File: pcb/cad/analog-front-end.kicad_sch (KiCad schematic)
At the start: 30 parts

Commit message: specify components used in front-end, validation and power circuits, except resistors
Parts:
- C?: footprint (none) -> Capacitor_SMD:C_0805_2012Metric_Pad1.18x1.45mm_HandSolder; Manufacturer (none) -> Prosperity Dielectrics Co; Part Number (none) -> MA0805CG-331J-500PR
- R?: footprint Resistor_SMD:R_0603_1608Metric -> Resistor_SMD:R_0603_1608Metric_Pad0.98x0.95mm_HandSolder; Vendor Link (none) -> https://www.digikey.com/en/products/detail/ERA-3AEB473V/P47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
- RV?: footprint (none) -> Potentiometer_SMD:Potentiometer_Bourns_3224X_Vertical; Manufacturer (none) -> Bourns; Part Number (none) -> 3224X-1-502E
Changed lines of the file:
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@@
       (effects (font (size 1.27 1.27)) (justify left))
     )
-    (property "Footprint" "" (id 2) (at 100.0252 67.31 0)
-      (effects (font (size 1.27 1.27)) hide)
-    )
-    (property "Datasheet" "~" (id 3) (at 99.06 63.5 0)
+    (property "Footprint" "Capacitor_SMD:C_0805_2012Metric_Pad1.18x1.45mm_HandSolder" (id 2) (at 100.0252 67.31 0)
+      (effects (font (size 1.27 1.27)) hide)
+    )
+    (property "Datasheet" "https://download.datasheets.com/pdfs/2015/3/22/4/27/47/982/pdc_/manual/ma0603cg-151j-500prg.pdf" (id 3) (at 99.06 63.5 0)
+      (effects (font (size 1.27 1.27)) hide)
+    )
+    (property "Description" "Ceramic Capacitor 330 pF 50V 5% SMD 0805 NPO" (id 4) (at 99.06 63.5 0)
+      (effects (font (size 1.27 1.27)) hide)
+    )
+    (property "Manufacturer" "Prosperity Dielectrics Co" (id 5) (at 99.06 63.5 0)
+      (effects (font (size 1.27 1.27)) hide)
+    )
+    (property "Part Number" "MA0805CG-331J-500PR" (id 6) (at 99.06 63.5 0)
       (effects (font (size 1.27 1.27)) hide)
     )
@@
       (effects (font (size 1.27 1.27)) (justify right))
     )
-    (property "Footprint" "" (id 2) (at 58.42 148.59 0)
-      (effects (font (size 1.27 1.27)) hide)
-    )
-    (property "Datasheet" "~" (id 3) (at 58.42 148.59 0)
+    (property "Footprint" "Potentiometer_SMD:Potentiometer_Bourns_3224X_Vertical" (id 2) (at 58.42 148.59 0)
+      (effects (font (size 1.27 1.27)) hide)
+    )
+    (property "Datasheet" "https://www.bourns.com/docs/Product-Datasheets/3224.pdf" (id 3) (at 58.42 148.59 0)
+      (effects (font (size 1.27 1.27)) hide)
+    )
+    (property "Manufacturer" "Bourns" (id 4) (at 58.42 148.59 0)
+      (effects (font (size 1.27 1.27)) hide)
+    )
+    (property "Part Number" "3224X-1-502E" (id 5) (at 58.42 148.59 0)
       (effects (font (size 1.27 1.27)) hide)
     )
@@
     (property "Reference" "R?" (id 0) (at 240.03 43.18 90))
     (property "Value" "47k" (id 1) (at 240.03 45.72 90))
-    (property "Footprint" "Resistor_SMD:R_0603_1608Metric" (id 2) (at 240.284 48.514 90)
+    (property "Footprint" "Resistor_SMD:R_0603_1608Metric_Pad0.98x0.95mm_HandSolder" (id 2) (at 240.284 48.514 90)
       (effects (font (size 1.27 1.27)) hide)
     )
@@
       (effects (font (size 1.27 1.27)) hide)
     )
+    (property "Description" "Resistor 47k 0.1% 0.1W SMD 0603" (id 7) (at 240.03 49.53 0)
+      (effects (font (size 1.27 1.27)) hide)
+    )
+    (property "Vendor Link" "https://www.digikey.com/en/products/detail/ERA-3AEB473V/P47KDBCT-ND/1466092" (id 8) (at 240.03 49.53 0)
+      (effects (font (size 1.27 1.27)) hide)
+    )

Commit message: create schematic for trigger aggregation, indication and actuation circuits
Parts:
- U? (x3): Part Number (none) -> LM393N
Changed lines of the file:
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@@
+      (effects (font (size 1.27 1.27)) hide)
+    )
+    (property "Part Number" "LM393N" (id 4) (at 93.98 142.24 0)
       (effects (font (size 1.27 1.27)) hide)
     )
@@
       (effects (font (size 1.27 1.27)) hide)
     )
+    (property "Part Number" "LM393N" (id 4) (at 93.98 154.94 0)
+      (effects (font (size 1.27 1.27)) hide)
+    )
     (pin "1")
     (pin "2")
@@
       (effects (font (size 1.27 1.27)) hide)
     )
+    (property "Part Number" "LM393N" (id 4) (at 135.89 179.07 0)
+      (effects (font (size 1.27 1.27)) hide)
+    )

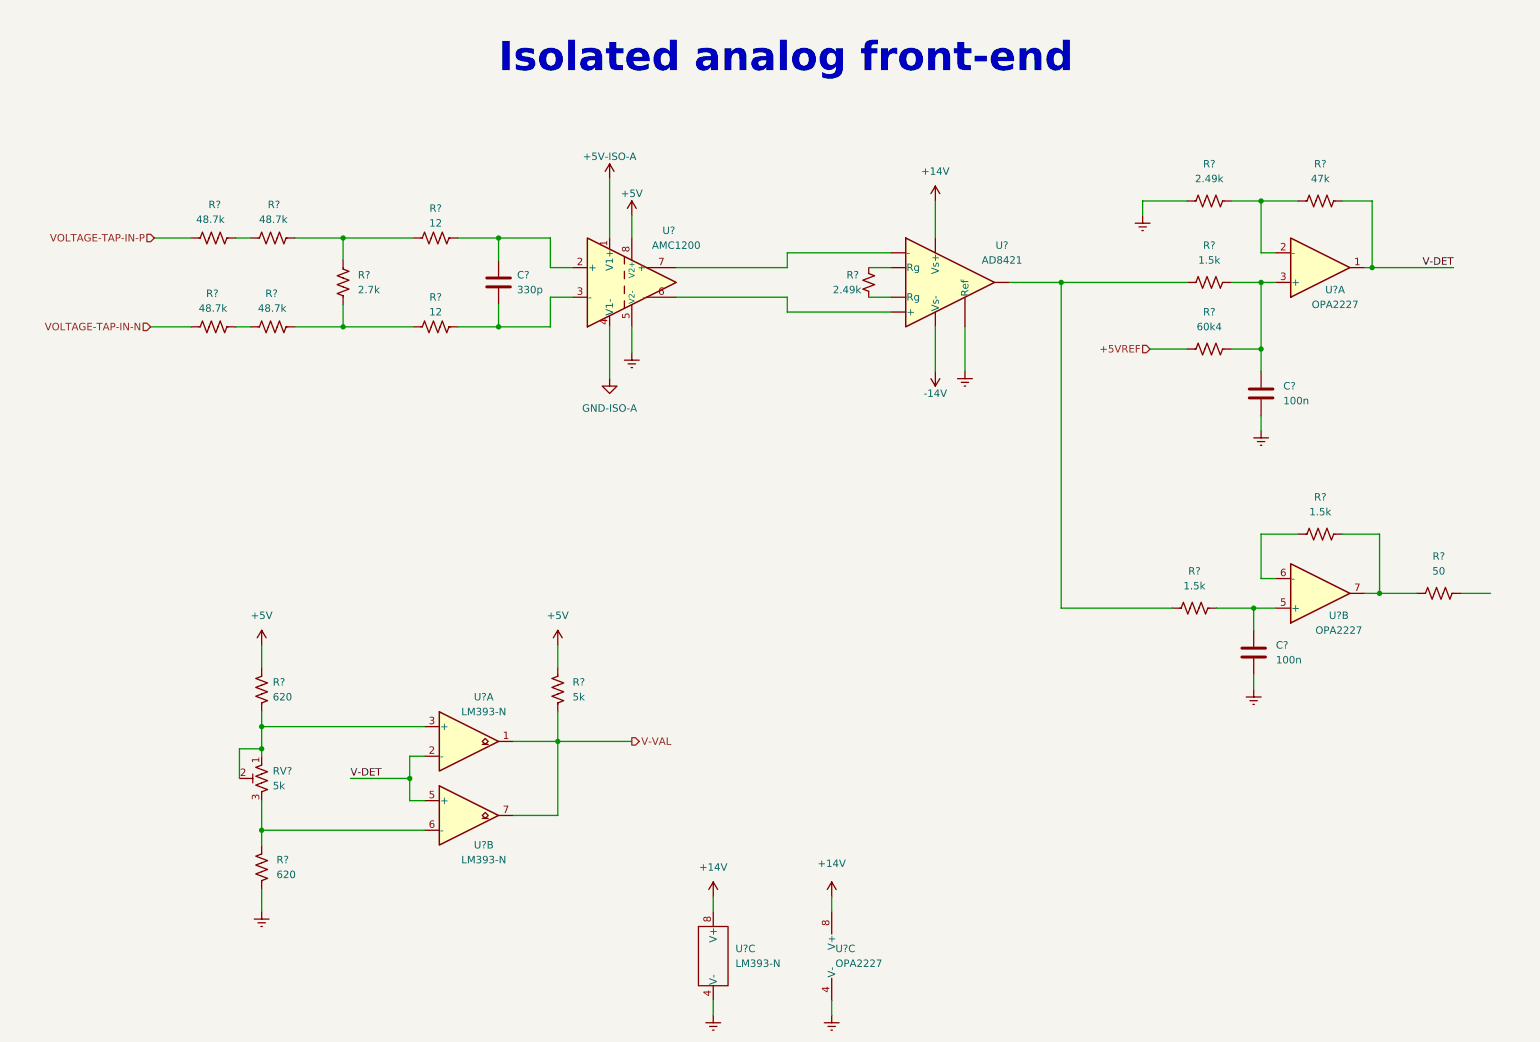
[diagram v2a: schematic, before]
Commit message: Created hierarchy connections, updates on analog-front-end and included 5V reference circuit
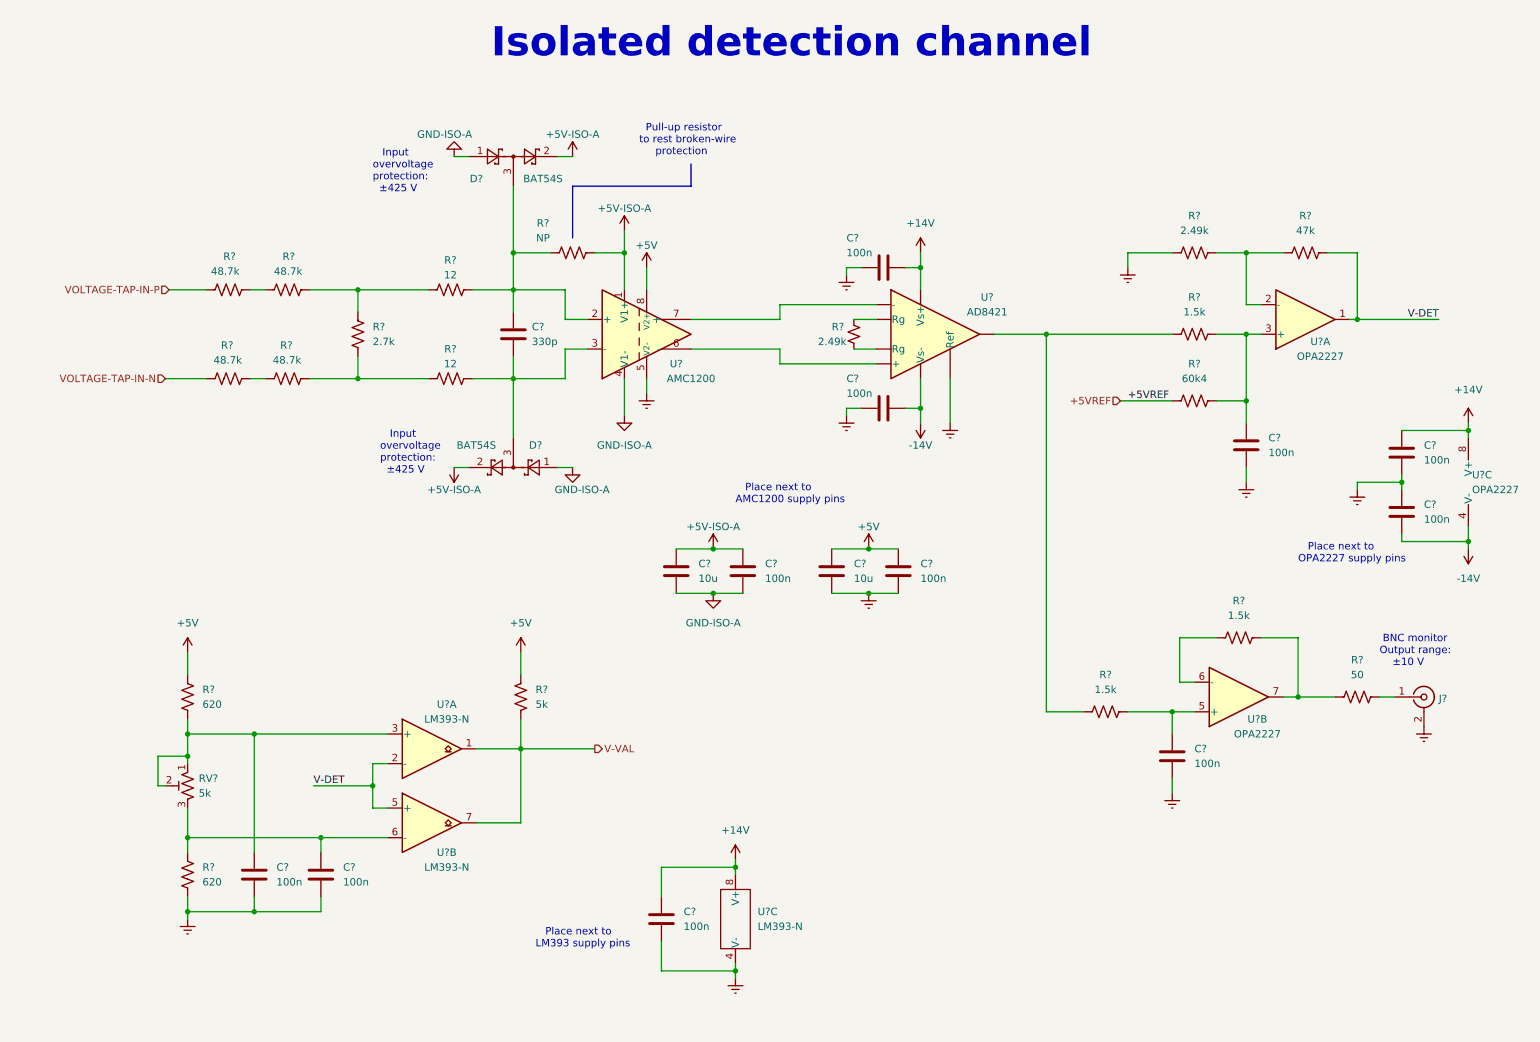
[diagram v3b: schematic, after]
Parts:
- removed R? (x2): 620, symbol Device:R_US
- added C? (x9): 100n, Capacitor_SMD:C_0603_1608Metric_Pad1.08x0.95mm_HandSolder, symbol Device:C
- added C? (x2): 10u, Capacitor_SMD:C_0805_2012Metric_Pad1.18x1.45mm_HandSolder, symbol Device:C
- added D? (x2): BAT54S, Package_TO_SOT_SMD:SOT-23, symbol Diode:BAT54S
- added J?: Conn_Coaxial, symbol Connector:Conn_Coaxial
- added R? (x2): 620, Resistor_SMD:R_0805_2012Metric_Pad1.20x1.40mm_HandSolder, symbol Device:R_US
- added R?: NP, Resistor_SMD:R_0805_2012Metric_Pad1.20x1.40mm_HandSolder, symbol Device:R_US
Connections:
- net +14V: now also C?.1, C?.1, C?.1
- net +5V: now also C?.1, C?.1, R?.2
- net +5V-ISO-A: now also C?.1, C?.1, D?.2, D?.2, R?.2
- net -14V: now also U?.4 (V-), C?.1, C?.2
- net Earth: now also C?.1, C?.2, C?.2, C?.2, C?.2, C?.2, C?.2, C?.2, C?.2, J?.2 (Ext), R?.1; no longer U?.4 (V-)
- net GND-ISO-A: now also C?.2, C?.2, D?.1, D?.1
- net at C?.1, R?.2, U?.2 (+): now also D?.3, R?.1
- net at C?.2, R?.2, U?.3 (-): now also D?.3
- net at RV?.3, U?.6 (-): now also C?.1, R?.2
- net at R?.2: now also J?.1 (In)
- net at RV?.1, RV?.2, U?.3 (+): now also C?.1, R?.1
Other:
- note added: "BNC monitor Output range: ±10 V"
- note added: "Input overvoltage protection: ±425 V"
- note added: "Isolated detection channel"
- note added: "Place next to AMC1200 supply pins"
- note added: "Place next to LM393 supply pins"
- note added: "Place next to OPA2227 supply pins"
- note added: "Pull-up resistor to rest broken-wire protection"
- note removed: "Isolated analog front-end"
- moved on the sheet: C?, R?, RV?, U?, U?A, U?B, U?C
